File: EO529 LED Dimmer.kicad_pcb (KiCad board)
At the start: 2 copper layers, 76.2 x 45.7 mm, 47 parts, among them J1 VBat, Q1 BC639, Q2 BC639, Q3 BC639, Q4 BC639, U1 NE556, U2 NE556

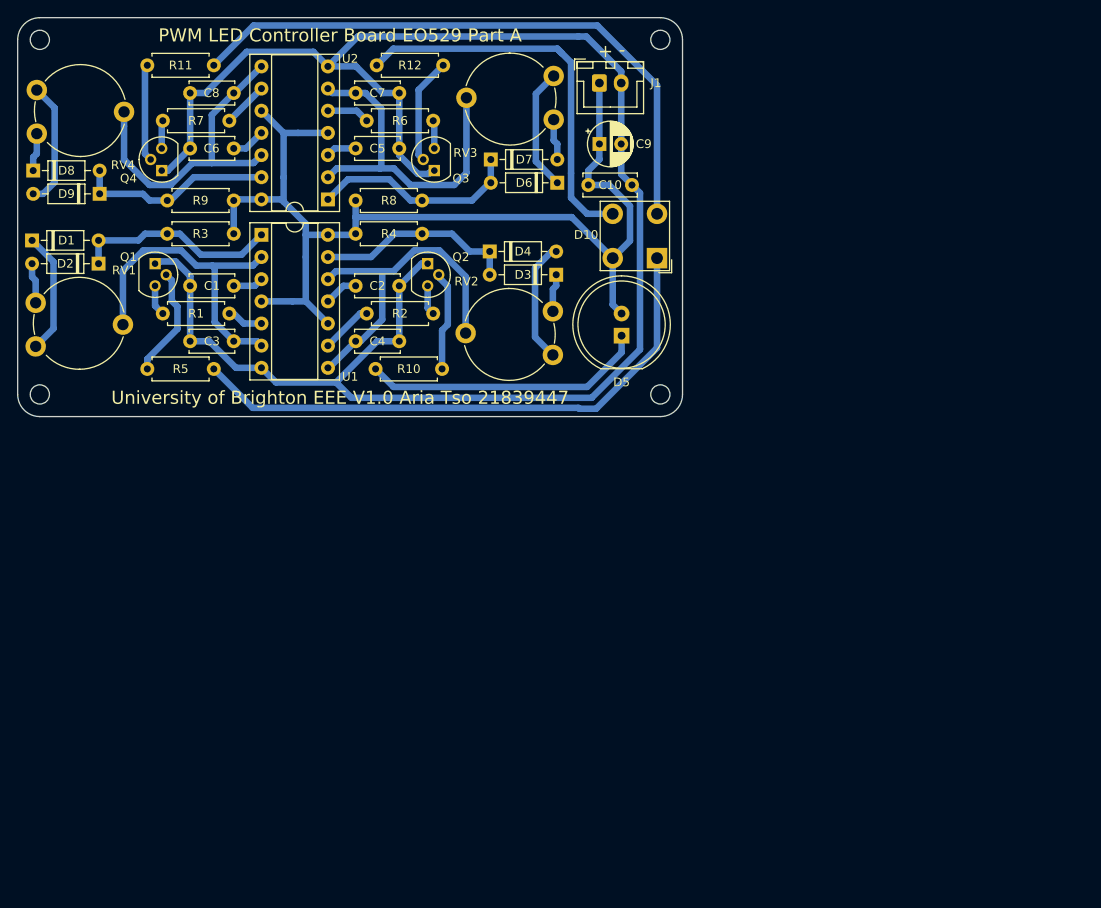
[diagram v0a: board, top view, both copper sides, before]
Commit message: Revision to circuit
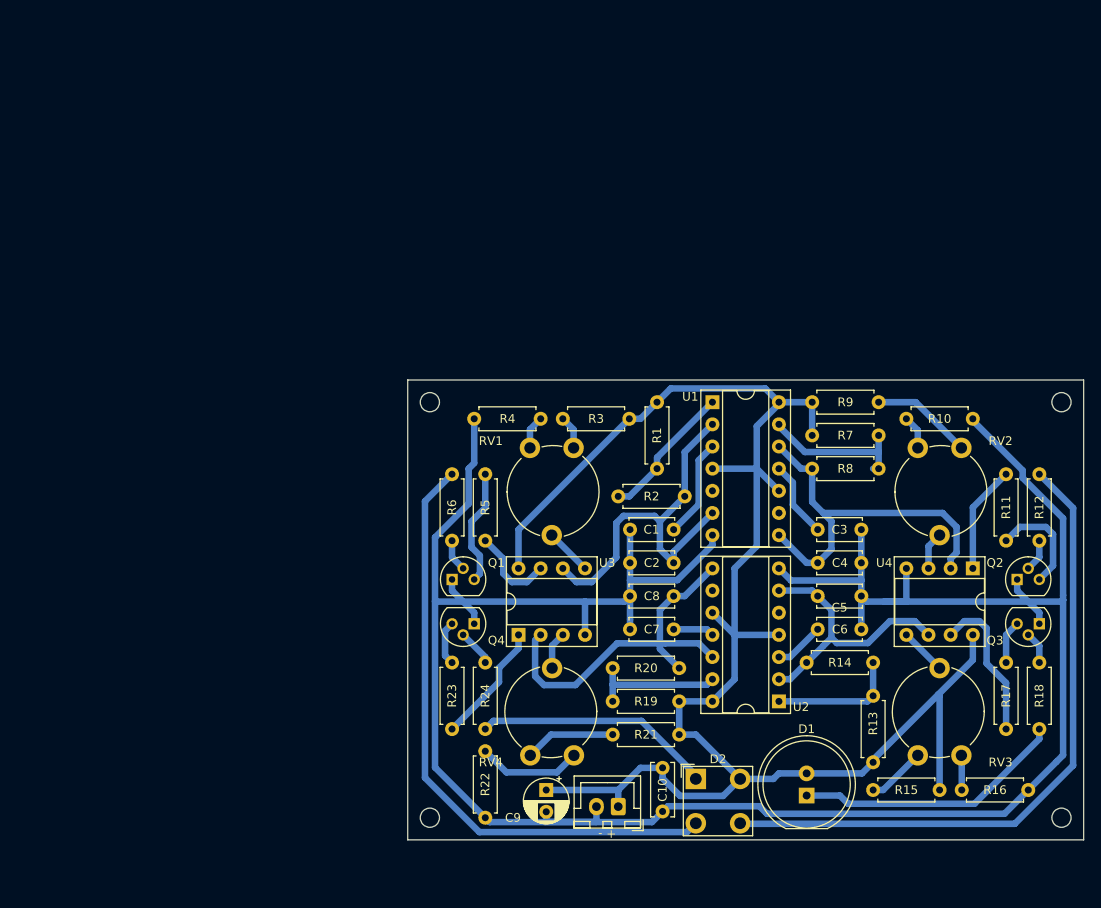
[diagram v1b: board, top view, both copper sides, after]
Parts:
- removed D10: LED_RGBA, LED_THT:LED_BL-FL7680RGB
- removed D3, D4, D6, D7, D8, D9: 1N4148, Diode_THT:D_DO-35_SOD27_P7.62mm_Horizontal
- removed D5: White, LED_THT:LED_D10.0mm
- added R13: 10k, Resistor_THT:R_Axial_DIN0207_L6.3mm_D2.5mm_P7.62mm_Horizontal, F.Cu at (118.1, 113.0)
- added R14: 10k, Resistor_THT:R_Axial_DIN0207_L6.3mm_D2.5mm_P7.62mm_Horizontal, F.Cu at (118.1, 101.6)
- added R15: 100k, Resistor_THT:R_Axial_DIN0207_L6.3mm_D2.5mm_P7.62mm_Horizontal, F.Cu at (125.7, 116.2)
- added R16: 100k, Resistor_THT:R_Axial_DIN0207_L6.3mm_D2.5mm_P7.62mm_Horizontal, F.Cu at (128.3, 116.2)
- added R17: 1k, Resistor_THT:R_Axial_DIN0207_L6.3mm_D2.5mm_P7.62mm_Horizontal, F.Cu at (133.3, 101.6)
- added R18: 180, Resistor_THT:R_Axial_DIN0207_L6.3mm_D2.5mm_P7.62mm_Horizontal, F.Cu at (137.2, 101.6)
- added R19: 10k, Resistor_THT:R_Axial_DIN0207_L6.3mm_D2.5mm_P7.62mm_Horizontal, F.Cu at (95.9, 106.0)
- added R20: 10k, Resistor_THT:R_Axial_DIN0207_L6.3mm_D2.5mm_P7.62mm_Horizontal, F.Cu at (88.3, 102.2)
- added R21: 100k, Resistor_THT:R_Axial_DIN0207_L6.3mm_D2.5mm_P7.62mm_Horizontal, F.Cu at (95.9, 109.9)
- added R22: 100k, Resistor_THT:R_Axial_DIN0207_L6.3mm_D2.5mm_P7.62mm_Horizontal, F.Cu at (73.7, 111.8)
- added R23: 1k, Resistor_THT:R_Axial_DIN0207_L6.3mm_D2.5mm_P7.62mm_Horizontal, F.Cu at (69.8, 101.6)
- added R24: 150, Resistor_THT:R_Axial_DIN0207_L6.3mm_D2.5mm_P7.62mm_Horizontal, F.Cu at (73.7, 101.6)
- added U3: LM393, Package_DIP:DIP-8_W7.62mm_Socket, F.Cu at (77.5, 98.4)
- added U4: LM393, Package_DIP:DIP-8_W7.62mm_Socket, F.Cu at (129.5, 90.8)
- D1: value 1N4148 -> White; footprint Diode_THT:D_DO-35_SOD27_P7.62mm_Horizontal -> LED_THT:LED_D10.0mm
- D2: value 1N4148 -> LED_RGBA; footprint Diode_THT:D_DO-35_SOD27_P7.62mm_Horizontal -> LED_THT:LED_BL-FL7680RGB
- R1, R2, R7, R8: value 1k -> 10k
- R10, R3, R4, R9: value 1k -> 100k
- R12: value 1k -> 220
- R5: value 180 -> 1k
- R6: value 10k -> 220
- moved R11 112.5 mm to (133.3, 87.6), turned to 90 degrees
- moved D1 109.2 mm to (110.5, 116.8), turned to 90 degrees
- moved RV4 94.2 mm to (83.8, 112.2), turned to 90 degrees
- moved RV3 90.8 mm to (128.2, 112.2), turned to 90 degrees
- moved D2 90.4 mm to (97.8, 114.9), turned to 0 degrees
- moved R12 87.4 mm to (137.2, 87.6), turned to 90 degrees
- moved Q3 86.6 mm to (137.2, 97.2), turned to 180 degrees
- moved C6 84.3 mm to (111.8, 94.0), turned to 0 degrees
- moved J1 83.0 mm to (88.9, 118.1), turned to 180 degrees
- moved R7 82.7 mm to (111.1, 75.6)
- moved U2 77.3 mm to (107.3, 106.0)
- moved Q2 76.6 mm to (134.6, 92.1), turned to 0 degrees
- moved C8 76.6 mm to (95.2, 94.0)
- moved C5 76.4 mm to (111.8, 97.8)
- moved C9 74.3 mm to (80.6, 116.2), turned to 270 degrees
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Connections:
- D1 pad 2: Net-(D1-Pad2) -> VCC
- D2 pad 1: Net-(D1-Pad2) -> Red
- D2 pad 2: Net-(D2-Pad2) -> Green
- R1 pad 1: Net-(Q1-Pad3) -> VCC
- R10 pad 1: Net-(Q2-Pad2) -> Net-(R10-Pad1)
- R10 pad 2: Net-(D5-Pad1) -> GND
- R11 pad 1: Net-(Q4-Pad2) -> Net-(Q2-Pad3)
- R11 pad 2: Green -> Net-(R11-Pad2)
- R12 pad 1: Net-(Q3-Pad2) -> Net-(Q2-Pad2)
- R2 pad 1: Net-(Q2-Pad3) -> Net-(R1-Pad2)
- R2 pad 2: Net-(R2-Pad2) -> Net-(C2-Pad1)
- R3 pad 2: Net-(D1-Pad2) -> Net-(R3-Pad2)
- R4 pad 1: VCC -> Net-(R4-Pad1)
- R4 pad 2: Net-(D3-Pad2) -> GND
- R5 pad 1: Net-(Q1-Pad2) -> Net-(Q1-Pad3)
- R5 pad 2: Red -> Net-(R5-Pad2)
- R6 pad 1: Net-(Q3-Pad3) -> Net-(Q1-Pad2)
- R6 pad 2: Net-(R6-Pad2) -> Green
- R7 pad 1: Net-(Q4-Pad3) -> VCC
- R8 pad 1: VCC -> Net-(R7-Pad2)
- R8 pad 2: Net-(D6-Pad2) -> Net-(C4-Pad1)
- R9 pad 2: Net-(D8-Pad2) -> Net-(R9-Pad2)
- RV1 pad 1: Net-(D1-Pad1) -> Net-(R4-Pad1)
- RV1 pad 2: Net-(C3-Pad1) -> Net-(RV1-Pad2)
- RV1 pad 3: Net-(D2-Pad2) -> Net-(R3-Pad2)
- RV2 pad 1: Net-(D3-Pad1) -> Net-(R10-Pad1)
- RV2 pad 2: Net-(C4-Pad1) -> Net-(RV2-Pad2)
- RV2 pad 3: Net-(D4-Pad2) -> Net-(R9-Pad2)
- RV3 pad 2: Net-(C7-Pad1) -> Net-(RV3-Pad2)
- RV4 pad 2: Net-(C8-Pad1) -> Net-(RV4-Pad2)
- U1 pad 1: Net-(D1-Pad2) -> Net-(R1-Pad2)
- U1 pad 11: Net-(C2-Pad1) -> Net-(C3-Pad1)
- U1 pad 13: Net-(D3-Pad2) -> Net-(R7-Pad2)
- U1 pad 2: Net-(C3-Pad1) -> Net-(C2-Pad1)
- U1 pad 5: Net-(R1-Pad2) -> Net-(U1-Pad5)
- U1 pad 6: Net-(C3-Pad1) -> Net-(C2-Pad1)
- U1 pad 9: Net-(R2-Pad2) -> Net-(U1-Pad9)
- U2 pad 1: Net-(D6-Pad2) -> Net-(R13-Pad2)
- U2 pad 11: Net-(C6-Pad1) -> Net-(C7-Pad1)
- U2 pad 13: Net-(D8-Pad2) -> Net-(R19-Pad2)
- U2 pad 2: Net-(C7-Pad1) -> Net-(C6-Pad1)
- U2 pad 5: Net-(R6-Pad2) -> Net-(U2-Pad5)
- U2 pad 6: Net-(C7-Pad1) -> Net-(C6-Pad1)
- U2 pad 9: Net-(R7-Pad2) -> Net-(U2-Pad9)
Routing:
- net GND: track 210.0 -> 285.7 mm
- net VCC: track 119.5 -> 194.7 mm
- net Net-(C2-Pad1): track 3.91 -> 44.1 mm
- net Red: track 65.9 -> 27.5 mm
- net Net-(C7-Pad1): track 40.2 -> 4.71 mm
- net Net-(D5-Pad1): track 32.6 -> 0.00 mm
- net Blue: track 44.4 -> 75.9 mm
- net Net-(C3-Pad1): track 37.2 -> 8.83 mm
- net Net-(C6-Pad1): track 3.91 -> 31.2 mm
- net Net-(D6-Pad2): track 24.0 -> 0.00 mm
- net Net-(D1-Pad2): track 23.6 -> 0.00 mm
- net Net-(D3-Pad2): track 23.2 -> 0.00 mm
- net Net-(D8-Pad2): track 22.6 -> 0.00 mm
- net Net-(R17-Pad2): track 0.00 -> 17.6 mm
- net Net-(D1-Pad1): track 14.0 -> 31.3 mm
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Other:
- board size 76.2 x 45.7 mm -> 77.5 x 52.7 mm
- board text added: "- +"
- board text removed: "+ -"
- board text removed: "PWM LED Controller Board EO529 Part A"
- board text removed: "University of Brighton EEE V1.0 Aria Tso 21839447"

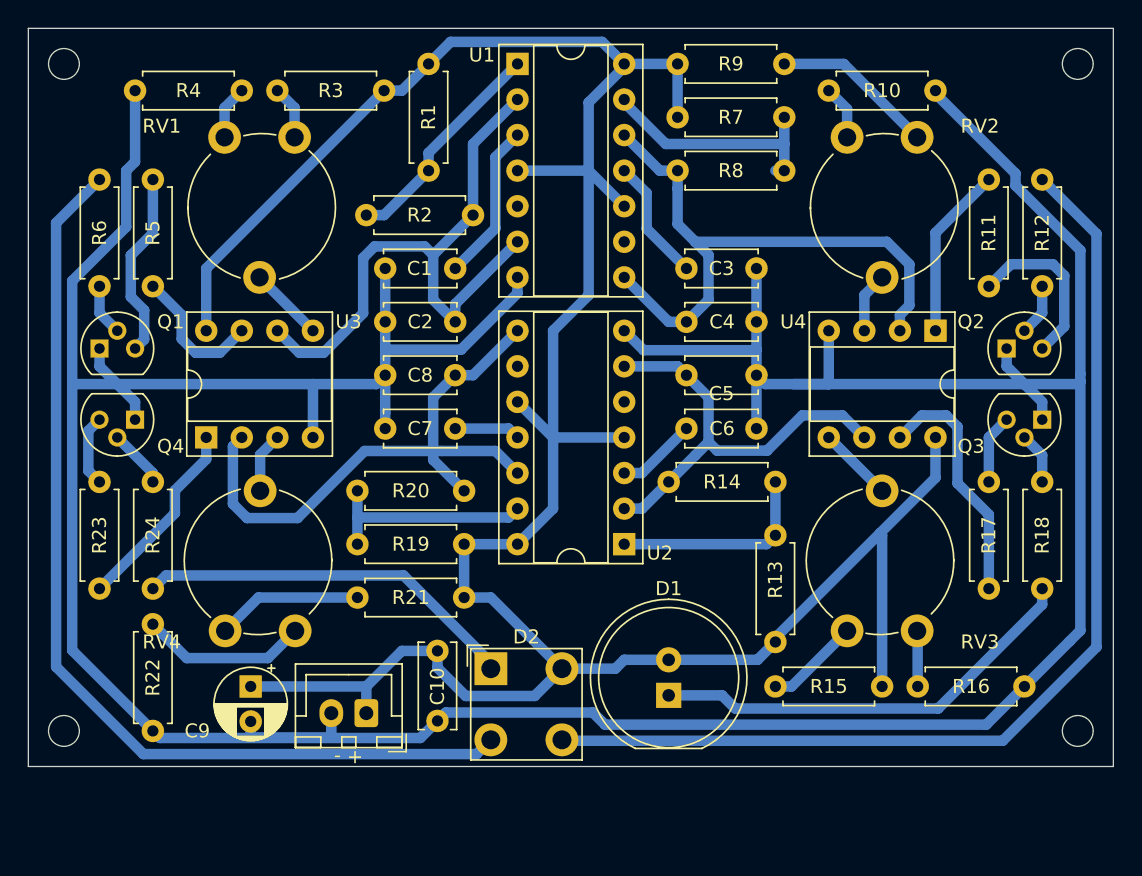
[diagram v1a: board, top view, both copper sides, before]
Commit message: Updated working design
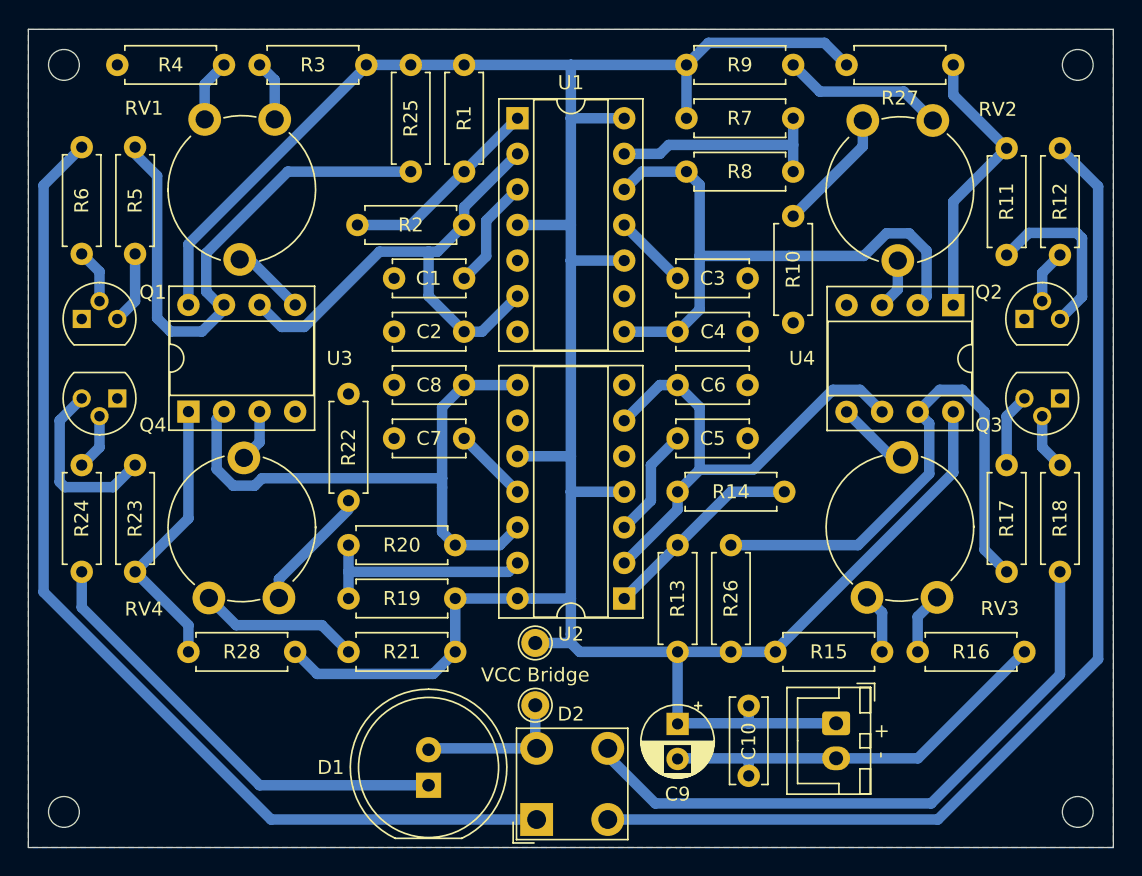
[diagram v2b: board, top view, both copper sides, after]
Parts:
- added R25: 1M, Resistor_THT:R_Axial_DIN0207_L6.3mm_D2.5mm_P7.62mm_Horizontal, F.Cu at (92.1, 79.4)
- added R26: 1M, Resistor_THT:R_Axial_DIN0207_L6.3mm_D2.5mm_P7.62mm_Horizontal, F.Cu at (114.9, 106.1)
- added R27: 1M, Resistor_THT:R_Axial_DIN0207_L6.3mm_D2.5mm_P7.62mm_Horizontal, F.Cu at (130.8, 71.8)
- added R28: 1M, Resistor_THT:R_Axial_DIN0207_L6.3mm_D2.5mm_P7.62mm_Horizontal, F.Cu at (76.2, 113.7)
- added TP1: TestPoint, TestPoint:TestPoint_THTPad_D2.0mm_Drill1.0mm, F.Cu at (101.0, 117.5)
- added TP2: TestPoint, TestPoint:TestPoint_THTPad_D2.0mm_Drill1.0mm, F.Cu at (101.0, 113.1)
- R10, R15, R16, R21, R22, R3, R4, R9: value 100k -> 82k
- R24: value 150 -> 180
- R6: value 220 -> 150
- moved J1 33.6 mm to (122.4, 118.8), turned to -90 degrees
- moved C9 30.6 mm to (111.1, 118.9)
- moved C10 22.6 mm to (116.2, 117.6)
- moved D1 18.3 mm to (93.3, 123.3)
- moved R22 16.5 mm to (87.6, 102.9), turned to 90 degrees
- moved D2 11.3 mm to (101.1, 125.7), turned to 90 degrees
- moved R10 9.31 mm to (119.4, 82.6), turned to -90 degrees
- moved R15 8.01 mm to (118.1, 113.7), turned to 0 degrees
- moved R13 7.02 mm to (111.1, 113.7)
- moved H2 5.78 mm to (67.3, 125.2)
- moved H4 5.78 mm to (139.7, 125.2)
- moved R5 5.46 mm to (72.4, 85.3), turned to 90 degrees
- moved R24 5.22 mm to (68.6, 100.4)
- moved R19 3.93 mm to (95.2, 109.9)
- moved R20 3.93 mm to (87.6, 106.1)
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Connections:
- D1 pad 1: Net-(D1-Pad1) -> Net-(R24-Pad2)
- D1 pad 2: VCC -> V_LED
- D2 pad 4: VCC -> V_LED
- R12 pad 2: Blue -> Green
- R18 pad 2: Net-(D1-Pad1) -> Blue
- R24 pad 2: Red -> Net-(R24-Pad2)
- R6 pad 2: Green -> Red
- U1 pad 5: Net-(U1-Pad5) -> unconnected-(U1-Pad5)
- U1 pad 9: Net-(U1-Pad9) -> unconnected-(U1-Pad9)
- U2 pad 5: Net-(U2-Pad5) -> unconnected-(U2-Pad5)
- U2 pad 9: Net-(U2-Pad9) -> unconnected-(U2-Pad9)
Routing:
- net GND: track 285.7 -> 29.2 mm
- net Red: track 27.5 -> 74.8 mm
- net Net-(R24-Pad2): track 0.00 -> 32.6 mm
- net Net-(D1-Pad1): track 31.3 -> 0.00 mm
- net Blue: track 75.9 -> 45.4 mm
- net Net-(U3-Pad7): track 9.96 -> 39.8 mm
- net Net-(U4-Pad7): track 17.6 -> 39.2 mm
- net V_LED: track 0.00 -> 10.9 mm
- net VCC: track 194.7 -> 204.5 mm
- net Net-(Q1-Pad3): track 13.4 -> 5.17 mm
- net Net-(R11-Pad2): track 12.4 -> 20.3 mm
- net Net-(Q4-Pad3): track 5.11 -> 12.8 mm
- net Net-(C2-Pad1): track 44.1 -> 36.6 mm
- net Green: track 70.1 -> 77.4 mm
- net Net-(R23-Pad2): track 14.0 -> 20.0 mm
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- added copper zone on B.Cu, net GND
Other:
- board size 77.5 x 52.7 mm -> 77.5 x 58.4 mm
- net class Default removed
- rule pad_to_mask_clearance: 0.05 -> 0
- board text added: "VCC Bridge"
